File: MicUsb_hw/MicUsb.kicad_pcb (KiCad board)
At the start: 2 copper layers, 61 x 44 mm, 80 parts, among them Q1 DVIUC6-4SC6, SW1 BUTTON

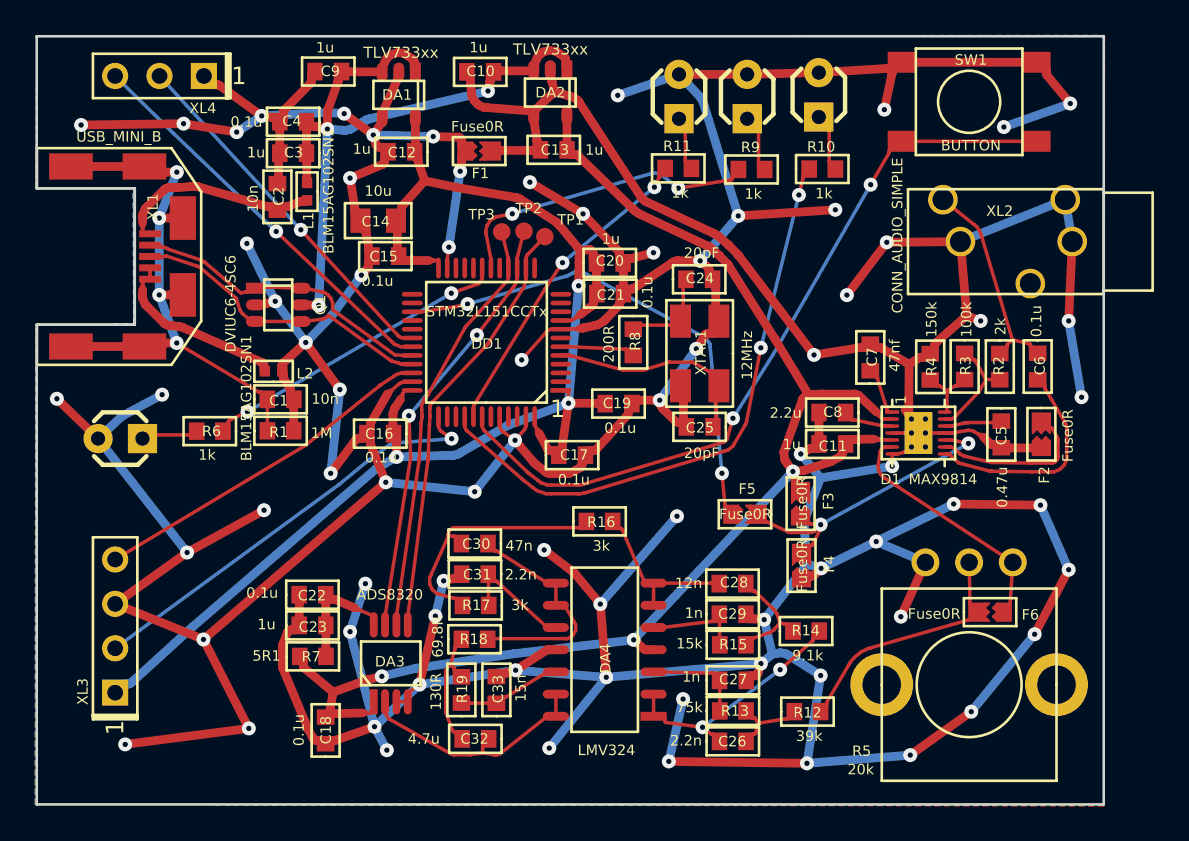
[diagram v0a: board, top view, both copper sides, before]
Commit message: plot again
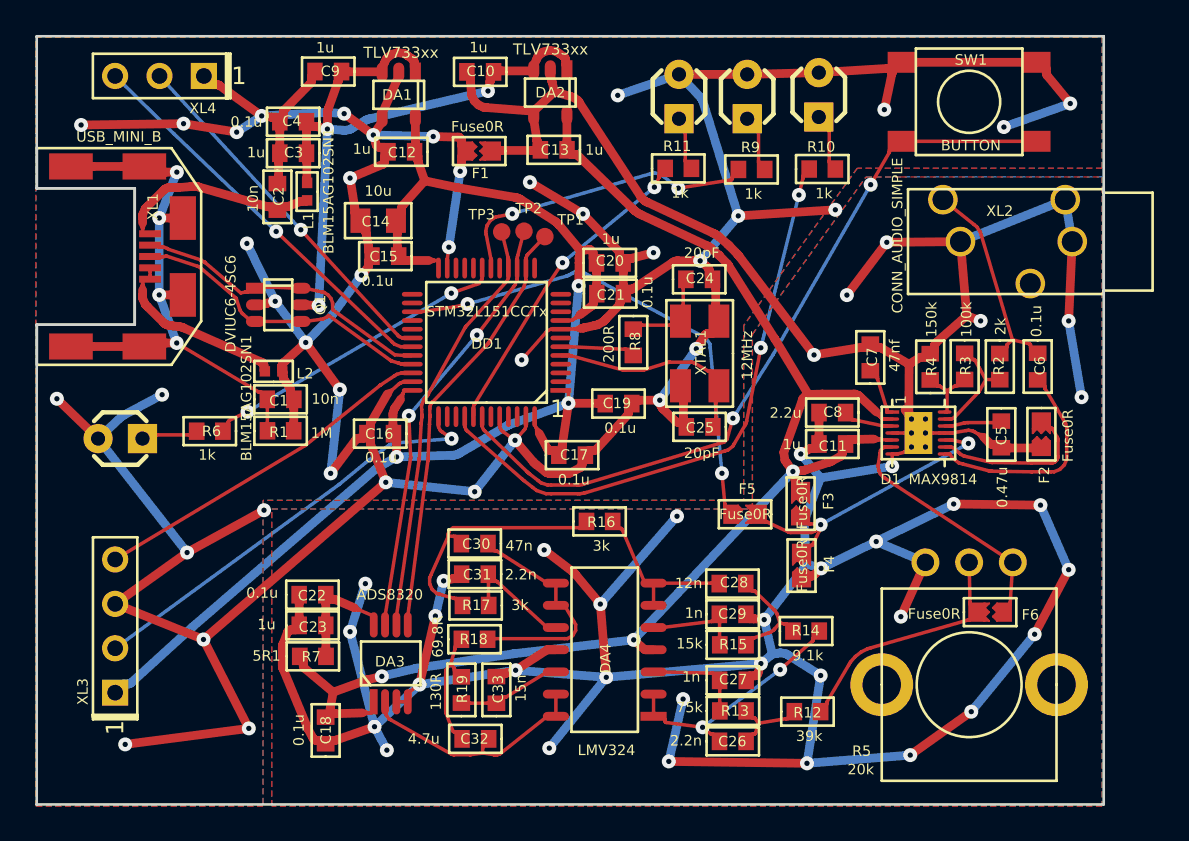
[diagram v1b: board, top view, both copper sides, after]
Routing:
- added copper zone on B.Cu, net AGND
- added copper zone on F.Cu, net AGND
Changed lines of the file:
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@@
   (general
     (links 193)
-    (no_connects 5)
-    (area 99.949999 77.755 169.174011 122.500001)
+    (no_connects 0)
+    (area 99.949999 78.24346 169.174011 122.500001)
     (thickness 1.6)
     (drawings 30)
@@
   (page A4)
   (layers
-    (0 F.Cu signal hide)
-    (31 B.Cu signal hide)
+    (0 F.Cu signal)
+    (31 B.Cu signal)
     (32 B.Adhes user)
     (33 F.Adhes user)
@@
     (visible_elements 7FFFF7FF)
     (pcbplotparams
-      (layerselection 0x00030_80000001)
-      (usegerberextensions false)
+      (layerselection 0x010e0_80000001)
+      (usegerberextensions true)
       (excludeedgelayer true)
       (linewidth 0.100000)
@@
       (outputformat 1)
       (mirror false)
-      (drillshape 1)
+      (drillshape 0)
       (scaleselection 1)
-      (outputdirectory ""))
+      (outputdirectory Gerber/))
   )
   (net 0 "")
@@
     (connect_pads (clearance 0.3))
     (min_thickness 0.254)
-    (fill yes (arc_segments 16) (thermal_gap 0.508) (thermal_bridge_width 0.508))
+    (fill yes (arc_segments 32) (thermal_gap 0.3) (thermal_bridge_width 0.508))
     (polygon
       (pts
-        (xy 166.1 122.5) (xy 105 122.4) (xy 105.05 94.9) (xy 110.65 94.95) (xy 110.65 87.15)
-        (xy 105.05 87.15) (xy 105.05 78.45) (xy 166.15 78.45) (xy 166.1 122.5)
+        (xy 105 78.5) (xy 166 78.5) (xy 166 86) (xy 152 86) (xy 145.5 95)
+        (xy 145.5 105) (xy 118 105) (xy 118 122.5) (xy 105 122.5) (xy 105 95)
       )
     )
@@
     (connect_pads (clearance 0.3))
     (min_thickness 0.254)
-    (fill yes (arc_segments 16) (thermal_gap 0.508) (thermal_bridge_width 0.508))
+    (fill yes (arc_segments 32) (thermal_gap 0.3) (thermal_bridge_width 0.508))
     (polygon
       (pts
-        (xy 105 78.45) (xy 166.1 78.4) (xy 166.1 122.45) (xy 104.95 122.4) (xy 105 94.95)
-        (xy 110.6 94.9) (xy 110.55 87.15) (xy 105 87.15) (xy 105.05 78.45)
+        (xy 105 78.5) (xy 166 78.5) (xy 166 86) (xy 152 86) (xy 145.5 95)
+        (xy 145.5 105) (xy 118 105) (xy 118 122.5) (xy 105 122.5)
+      )
+    )
+  )
+  (zone (net 6) (net_name AGND) (layer F.Cu) (hatch edge 0.508)
+    (connect_pads (clearance 0.3))
+    (min_thickness 0.254)
+    (fill yes (arc_segments 32) (thermal_gap 0.3) (thermal_bridge_width 0.508))
+    (polygon
+      (pts
+        (xy 166 86.5) (xy 166 122.5) (xy 118.5 122.5) (xy 118.5 105.5) (xy 146 105.5)
+        (xy 146 95.5) (xy 152.5 86.5) (xy 154.5 86.5)
+      )
+    )
+  )
+  (zone (net 6) (net_name AGND) (layer B.Cu) (hatch edge 0.508)
+    (connect_pads (clearance 0.3))
+    (min_thickness 0.254)
+    (fill yes (arc_segments 32) (thermal_gap 0.3) (thermal_bridge_width 0.508))
+    (polygon
+      (pts
+        (xy 166 86.5) (xy 166 122.5) (xy 118.5 122.5) (xy 118.5 105.5) (xy 146 105.5)
+        (xy 146 95.5) (xy 152.5 86.5)
       )
     )
